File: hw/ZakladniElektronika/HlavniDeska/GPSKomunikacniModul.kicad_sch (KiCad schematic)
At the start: 5 parts, among them J3 Conn_2Rows-75Pins

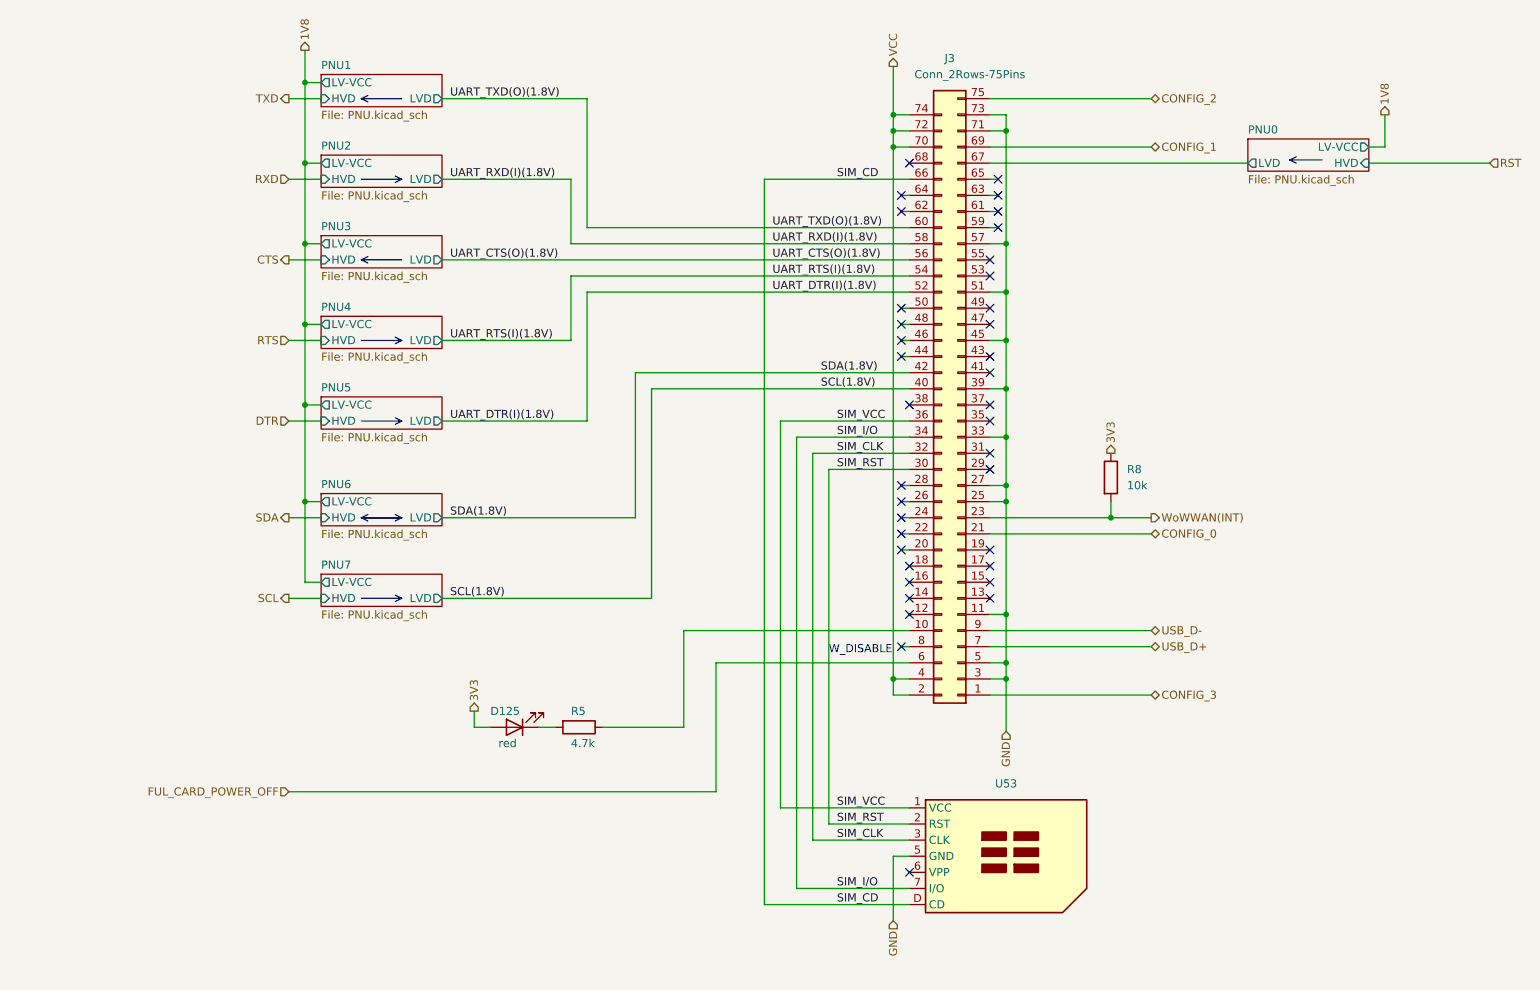
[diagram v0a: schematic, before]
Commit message: USB_multiplexer a přehlednost
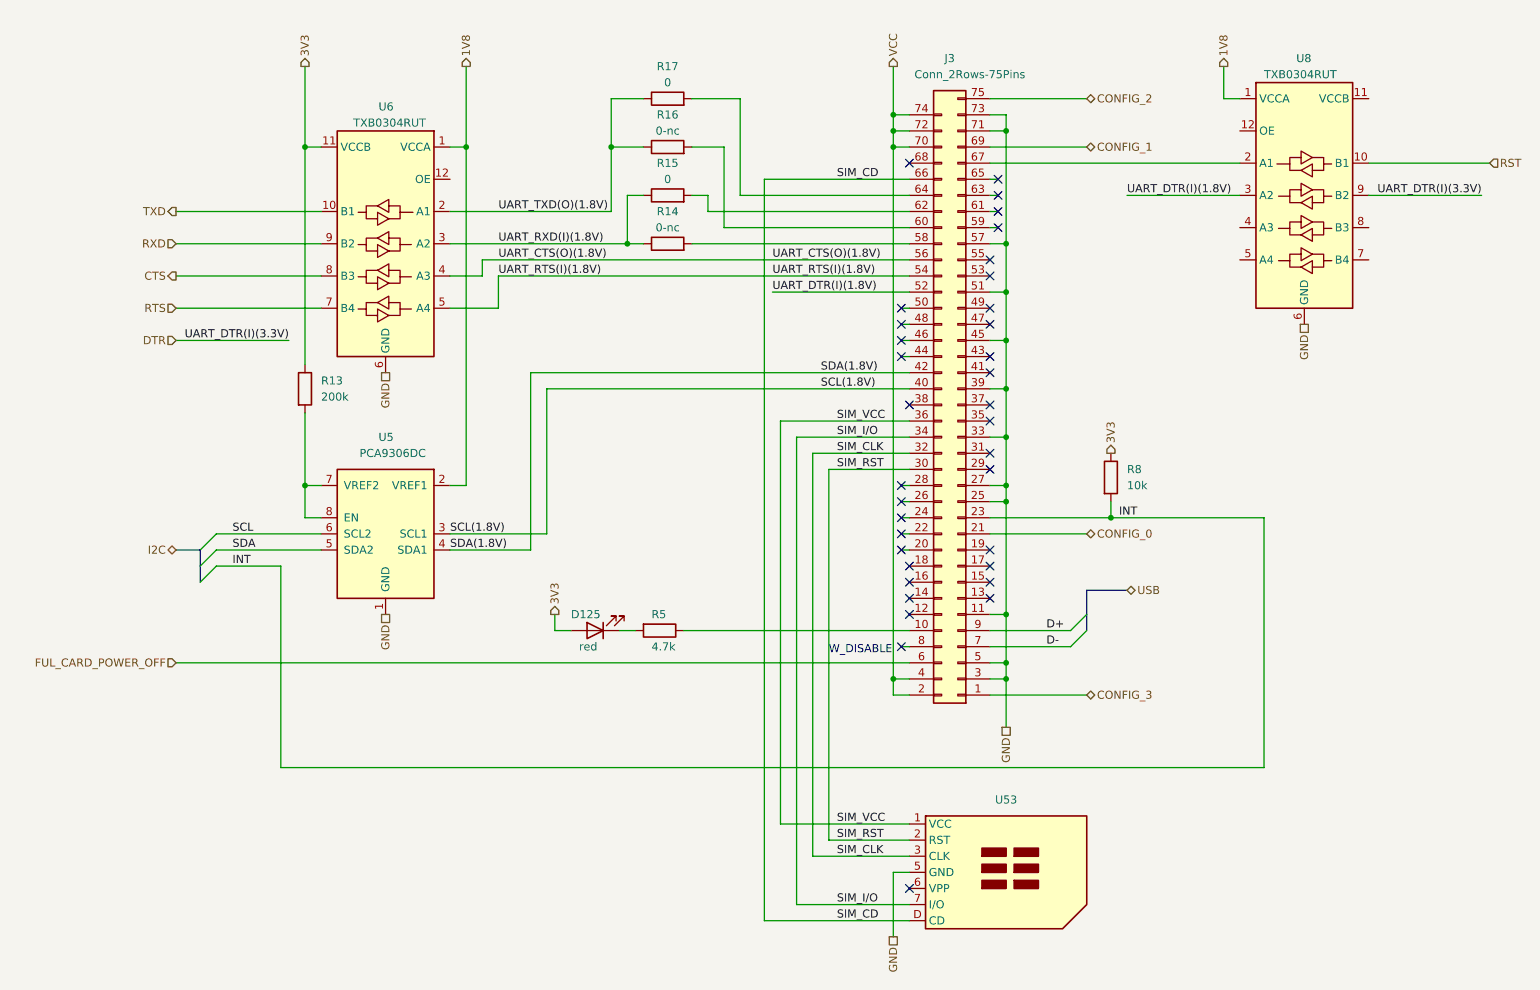
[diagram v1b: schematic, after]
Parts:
- added R13: 200k, Resistor_SMD:R_0402_1005Metric, symbol Device:R
- added R14, R16: 0-nc, symbol Device:R
- added R15, R17: 0, Resistor_SMD:R_0805_2012Metric_Pad1.20x1.40mm_HandSolder, symbol Device:R
- added U5: PCA9306DC, Package_SO:VSSOP-8_2.3x2mm_P0.5mm, symbol Interface:PCA9306DC
- added U6, U8: TXB0304RUT, Package_DFN_QFN:Texas_R-PUQFN-N12, symbol Logic_LevelTranslator:TXB0304RUT
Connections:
- net 1V8: now also U5.2 (VREF1), U6.1 (VCCA), U8.1 (VCCA)
- net 3V3: now also R13.1, U6.11 (VCCB)
- net CTS: now also U6.8 (B3)
- net DTR: now also U8.9 (B2)
- net GND: now also U5.1 (GND), U6.6 (GND), U8.6 (GND)
- net RST: now also U8.10 (B1)
- net RTS: now also U6.7 (B4)
- net RXD: now also U6.9 (B2)
- net SCL: now also U5.6 (SCL2)
- net SCL(1.8V): now also U5.3 (SCL1)
- net SDA: now also U5.5 (SDA2)
- net SDA(1.8V): now also U5.4 (SDA1)
- net TXD: now also U6.10 (B1)
- net UART_CTS(O)(1.8V): now also U6.4 (A3)
- net UART_DTR(I)(1.8V): now also U8.3 (A2)
- net UART_RTS(I)(1.8V): now also U6.5 (A4)
- net UART_RXD(I)(1.8V): now also R14.1, R15.1, U6.3 (A2); no longer J3.58 (Pin_58)
- net UART_TXD(O)(1.8V): now also R16.1, R17.1, U6.2 (A1); no longer J3.60 (Pin_60)
- net at J3.62 (Pin_62): now also R15.2
- net at J3.64 (Pin_64): now also R17.2
- net PNU0/LVD: no longer names the net of J3.67 (Pin_67)
- net PNU0/LVD: now also U8.2 (A1)
- net USB_D+ renamed D-
- net USB_D- renamed D+
- net WoWWAN(INT) renamed INT
- new net: R13.2, U5.7 (VREF2), U5.8 (EN)
- new net: J3.60 (Pin_60), R16.2
- new net: J3.58 (Pin_58), R14.2
- no-connect marks 37 -> 35
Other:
- removed sheet PNU0
- removed sheet PNU1
- removed sheet PNU2
- removed sheet PNU3
- removed sheet PNU4
- removed sheet PNU5
- removed sheet PNU6
- removed sheet PNU7
- moved on the sheet: D125, R5, U53
